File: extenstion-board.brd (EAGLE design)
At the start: 91.4 x 73.3 mm, 13 parts

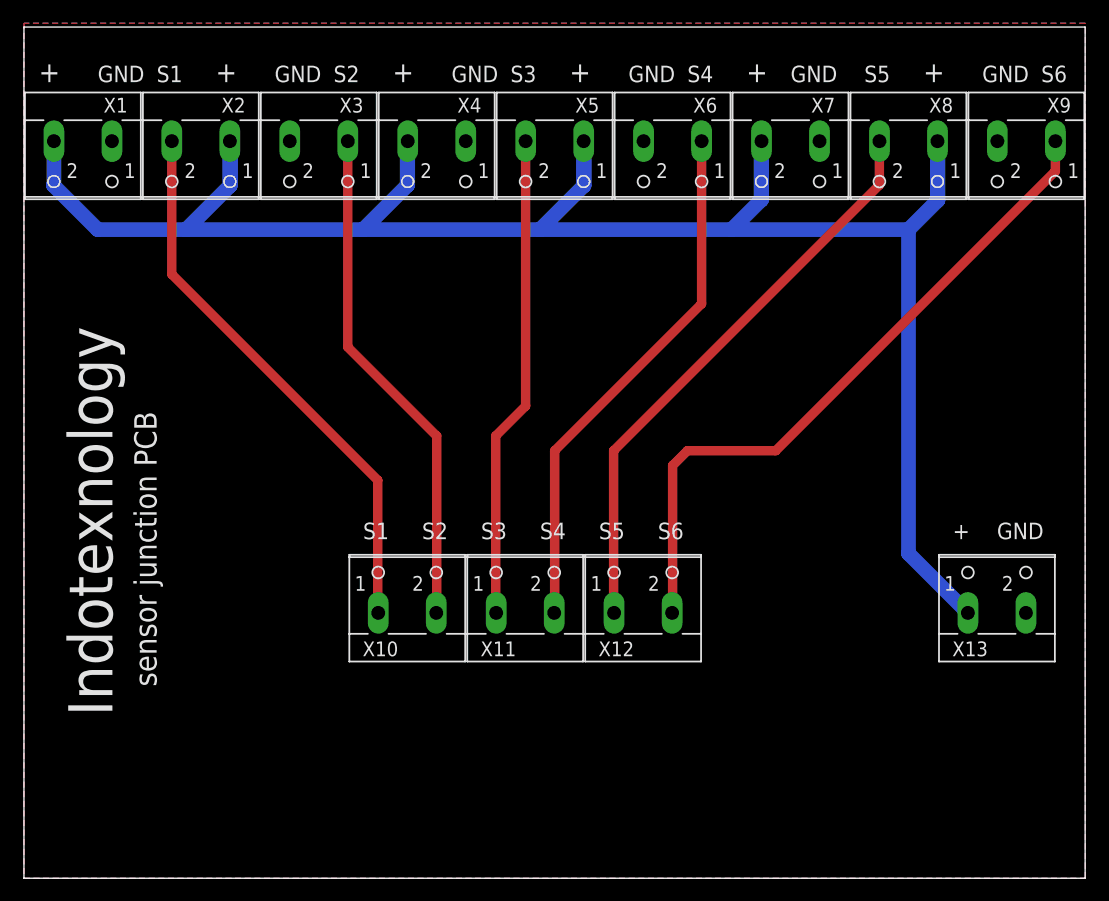
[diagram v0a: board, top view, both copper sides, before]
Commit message: added provision screw plug
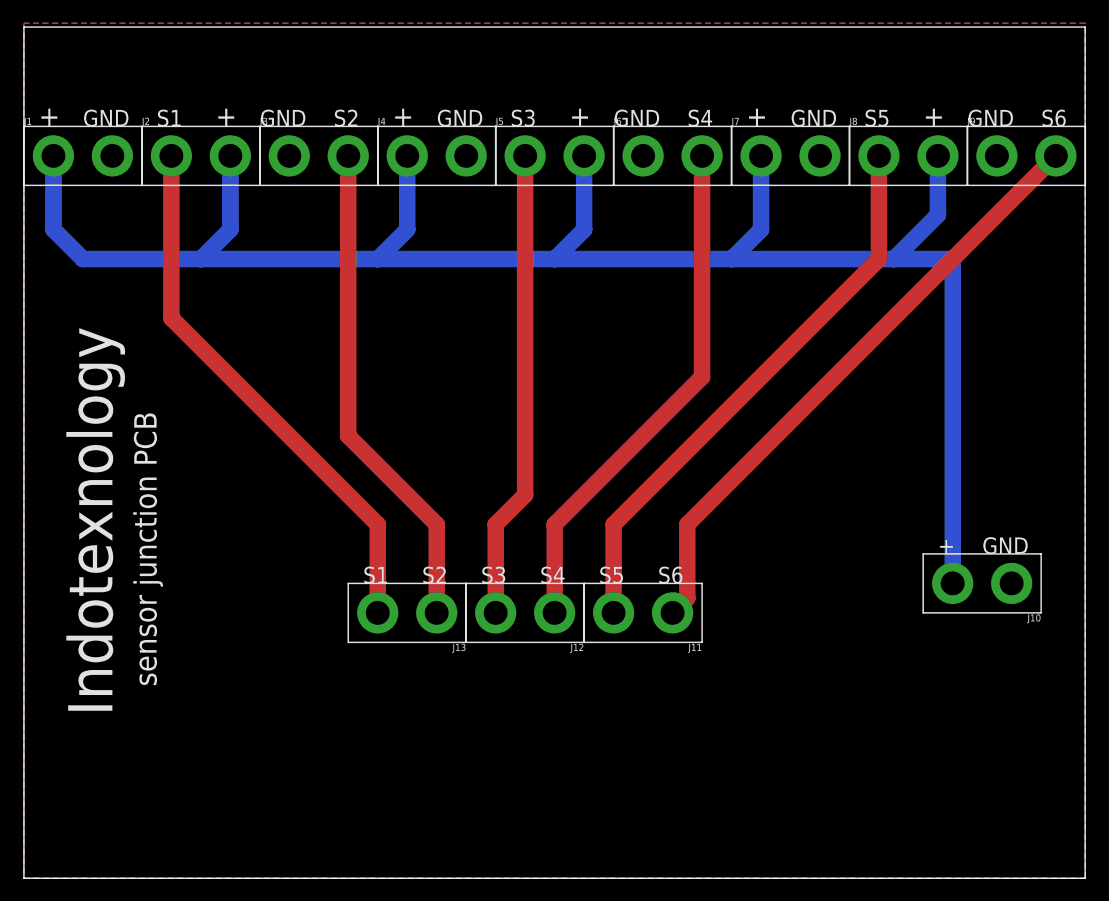
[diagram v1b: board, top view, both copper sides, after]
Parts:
- removed X1, X10, X11, X12, X13, X2, X3, X4, X5, X6, X7, X8, X9: (no value), con-wago-500:W237-102
- added J1, J10, J11, J12, J13, J2, J3, J4, J5, J6, J7, J8, J9: (no value), SparkFun-Connectors:1X02_XTRA_BIG
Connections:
- net +12V: now also J1.1, J10.2, J2.2, J4.1, J5.2, J7.1, J8.2; no longer X1.2, X13.1, X2.1, X4.2, X5.1, X7.2, X8.1
- net GND: now also J1.2, J10.1, J3.1, J4.2, J6.1, J7.2, J9.1; no longer X1.1, X13.2, X3.2, X4.1, X6.2, X7.1, X9.2
- net N$1: now also J11.2, J8.1; no longer X12.1, X8.2
- net N$2: now also J13.2, J2.1; no longer X10.1, X2.2
- net N$3: now also J13.1, J3.2; no longer X10.2, X3.1
- net N$4: now also J12.2, J5.1; no longer X11.1, X5.2
- net N$5: now also J12.1, J6.2; no longer X11.2, X6.1
- net N$6: now also J11.1, J9.2; no longer X12.2, X9.1
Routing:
- net +12V: track 181.0 -> 163.0 mm
- net N$6: track 58.8 -> 53.0 mm
- net N$1: track 50.1 -> 48.8 mm
- net N$4: track 41.7 -> 40.4 mm
- net N$3: track 43.8 -> 42.5 mm
- net N$5: track 45.9 -> 44.6 mm
- net N$2: track 48.0 -> 46.7 mm
